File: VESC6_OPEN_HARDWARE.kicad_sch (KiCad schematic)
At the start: 20 parts, among them P1 USB_OTG, P2 TS_CAN, P3 SWD, P4 HALL/Encoder, P5 TS_CAN, P7 Custom

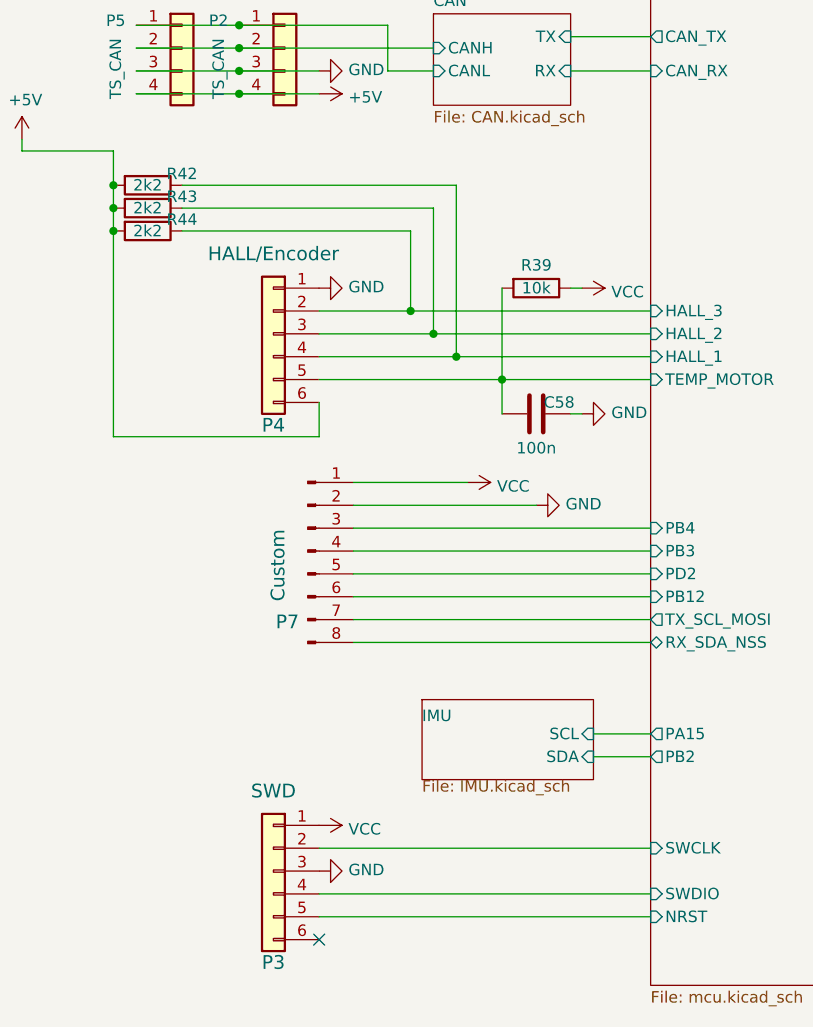
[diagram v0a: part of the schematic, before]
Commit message: Adjusted connectors and routing
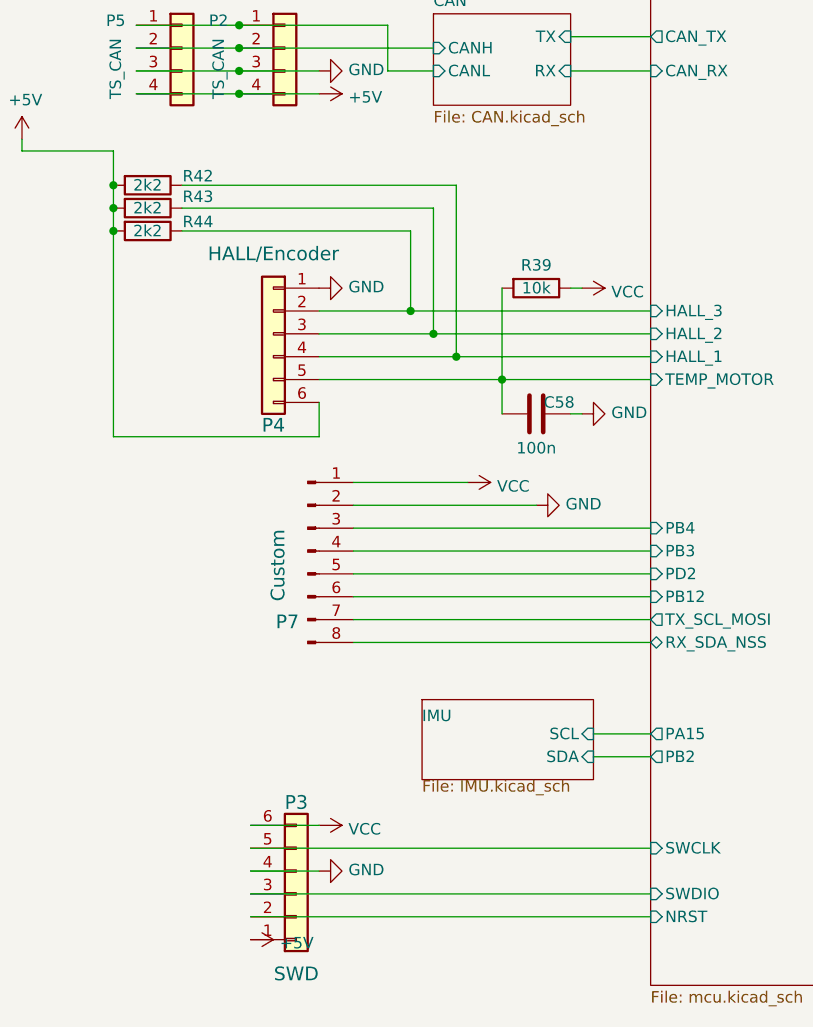
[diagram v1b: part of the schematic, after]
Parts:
- P3: footprint Connector_PinSocket_1.27mm:PinSocket_1x06_P1.27mm_Vertical -> Connector_JST:JST_SH_SM06B-SRSS-TB_1x06-1MP_P1.00mm_Horizontal
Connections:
- net +5V: now also P3.1 (Pin_1)
- net GND: now also P3.4 (Pin_4); no longer P3.3 (Pin_3)
- net VCC: now also P3.6 (Pin_6); no longer P3.1 (Pin_1)
- net stm32f40x/NRST: now also P3.2 (Pin_2); no longer P3.5 (Pin_5)
- net stm32f40x/SWCLK: now also P3.5 (Pin_5); no longer P3.2 (Pin_2)
- net stm32f40x/SWDIO: now also P3.3 (Pin_3); no longer P3.4 (Pin_4)
- no-connect marks 2 -> 1
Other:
- moved on the sheet: P3
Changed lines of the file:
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@@
 		(at 96.52 34.29)
 	)
-	(no_connect
-		(at 91.44 151.13)
-	)
 	(wire
 		(pts
@@
 	(wire
 		(pts
+			(xy 83.82 143.51) (xy 91.44 143.51)
+		)
+		(stroke
+			(width 0)
+			(type default)
+		)
+	)
+	(wire
+		(pts
 			(xy 99.06 49.53) (xy 99.06 54.61)
 		)
@@
 	(wire
 		(pts
+			(xy 83.82 138.43) (xy 91.44 138.43)
+		)
+		(stroke
+			(width 0)
+			(type default)
+		)
+	)
+	(wire
+		(pts
 			(xy 96.52 24.13) (xy 105.41 24.13)
 		)
@@
 	(wire
 		(pts
-			(xy 128.27 140.97) (xy 91.44 140.97)
+			(xy 128.27 140.97) (xy 83.82 140.97)
 		)
 		(stroke
@@
 	(wire
 		(pts
-			(xy 91.44 146.05) (xy 128.27 146.05)
+			(xy 83.82 146.05) (xy 128.27 146.05)
 		)
 		(stroke
@@
 	(wire
 		(pts
-			(xy 91.44 148.59) (xy 128.27 148.59)
+			(xy 83.82 148.59) (xy 128.27 148.59)
 		)
 		(stroke
@@
 		(dnp no)
 		(property "Reference" "R44"
-			(at 76.2 71.12 90)
+			(at 77.978 71.374 90)
 			(effects
 				(font
@@
 		(dnp no)
 		(property "Reference" "R43"
-			(at 76.2 68.58 90)
+			(at 77.978 68.58 90)
 			(effects
 				(font
@@
 		(dnp no)
 		(property "Reference" "R42"
-			(at 76.2 66.04 90)
+			(at 77.978 66.294 90)
 			(effects
 				(font
@@
 			)
 		)
-		(property "Datasheet" "https://datasheet.lcsc.com/lcsc/1811151141_Korean-Hroparts-Elec-U-D-M5DD-W-1_C145795.pdf"
+		(property "Datasheet" "https://www.molex.com/content/dam/molex/molex-dot-com/products/automated/en-us/salesdrawingpdf/482/48258/482580001_sd.pdf?"
 			(at 92.71 30.48 0)
 			(effects
@@
 	)
 	(symbol
+		(lib_id "power:+5V")
+		(at 83.82 151.13 270)
+		(unit 1)
+		(exclude_from_sim no)
+		(in_bom yes)
+		(on_board yes)
+		(dnp no)
+		(property "Reference" "#PWR0121"
+			(at 80.01 151.13 0)
+			(effects
+				(font
+					(size 1.27 1.27)
+				)
+				(hide yes)
+			)
+		)
+		(property "Value" "+5V"
+			(at 87.0712 151.511 90)
+			(effects
+				(font
+					(size 1.27 1.27)
+				)
+				(justify left)
+			)
+		)
+		(property "Footprint" ""
+			(at 83.82 151.13 0)
+			(effects
+				(font
+					(size 1.27 1.27)
+				)
+				(hide yes)
+			)
+		)
+		(property "Datasheet" ""
+			(at 83.82 151.13 0)
+			(effects
+				(font
+					(size 1.27 1.27)
+				)
+				(hide yes)
+			)
+		)
+		(property "Description" ""
+			(at 83.82 151.13 0)
+			(effects
+				(font
+					(size 1.27 1.27)
+				)
+			)
+		)
+		(pin "1"
+		)
+		(instances
+			(project "VESC6_OPEN_HARDWARE"
+				(path "/8bc2c25a-a1f1-4ce8-b96a-a4f8f4c35079"
+					(reference "#PWR0121")
+					(unit 1)
+				)
+			)
+		)
+	)
+	(symbol
 		(lib_id "power:GND")
 		(at 115.57 102.87 90)
@@
 	(symbol
 		(lib_id "Connector_Generic:Conn_01x06")
-		(at 86.36 143.51 0)
-		(mirror y)
+		(at 88.9 146.05 0)
+		(mirror x)
 		(unit 1)
 		(exclude_from_sim no)
@@
 		(dnp no)
 		(property "Reference" "P3"
-			(at 86.36 153.67 0)
+			(at 88.9 135.89 0)
 			(effects
 				(font
@@
 		)
 		(property "Value" "SWD"
-			(at 86.36 134.62 0)
+			(at 88.9 154.94 0)
 			(effects
 				(font
@@
 			)
 		)
-		(property "Footprint" "Connector_PinSocket_1.27mm:PinSocket_1x06_P1.27mm_Vertical"
-			(at 86.36 143.51 0)
+		(property "Footprint" "Connector_JST:JST_SH_SM06B-SRSS-TB_1x06-1MP_P1.00mm_Horizontal"
+			(at 88.9 146.05 0)
 			(effects
 				(font
@@
 		)
 		(property "Datasheet" "https://www.molex.com/content/dam/molex/molex-dot-com/products/automated/en-us/salesdrawingpdf/505/505567/5055670671_sd.pdf?inline"
-			(at 86.36 143.51 0)
+			(at 88.9 146.05 0)
 			(effects
 				(font
@@
 		)
 		(property "Description" ""
-			(at 86.36 143.51 0)
+			(at 88.9 146.05 0)
 			(effects
 				(font
@@
 		)
 		(property "LCSC part no." "C160405"
-			(at 86.36 143.51 0)
+			(at 88.9 146.05 0)
 			(effects
 				(font
@@
 		)
 		(property "Critical" "Y"
-			(at 86.36 143.51 0)
+			(at 88.9 146.05 0)
 			(effects
 				(font
@@
 		)
 		(property "Link" ""
-			(at 86.36 143.51 0)
+			(at 88.9 146.05 0)
 			(effects
 				(font
@@
 		)
 		(property "MFP" ""
-			(at 86.36 143.51 0)
+			(at 88.9 146.05 0)
 			(effects
 				(font
